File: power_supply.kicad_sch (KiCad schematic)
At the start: 16 parts, among them SW1 SW_DIP_x01, T1 1x230V 2x30V 300VA

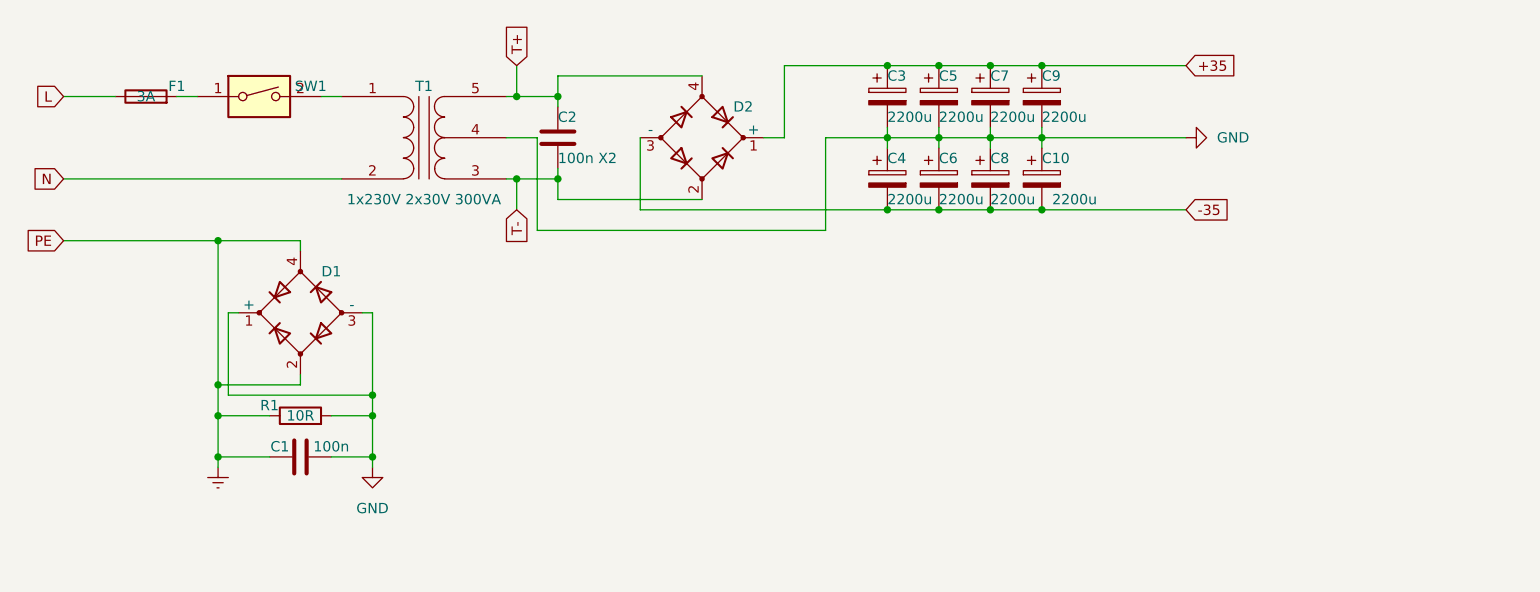
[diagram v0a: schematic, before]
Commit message: cosmetics
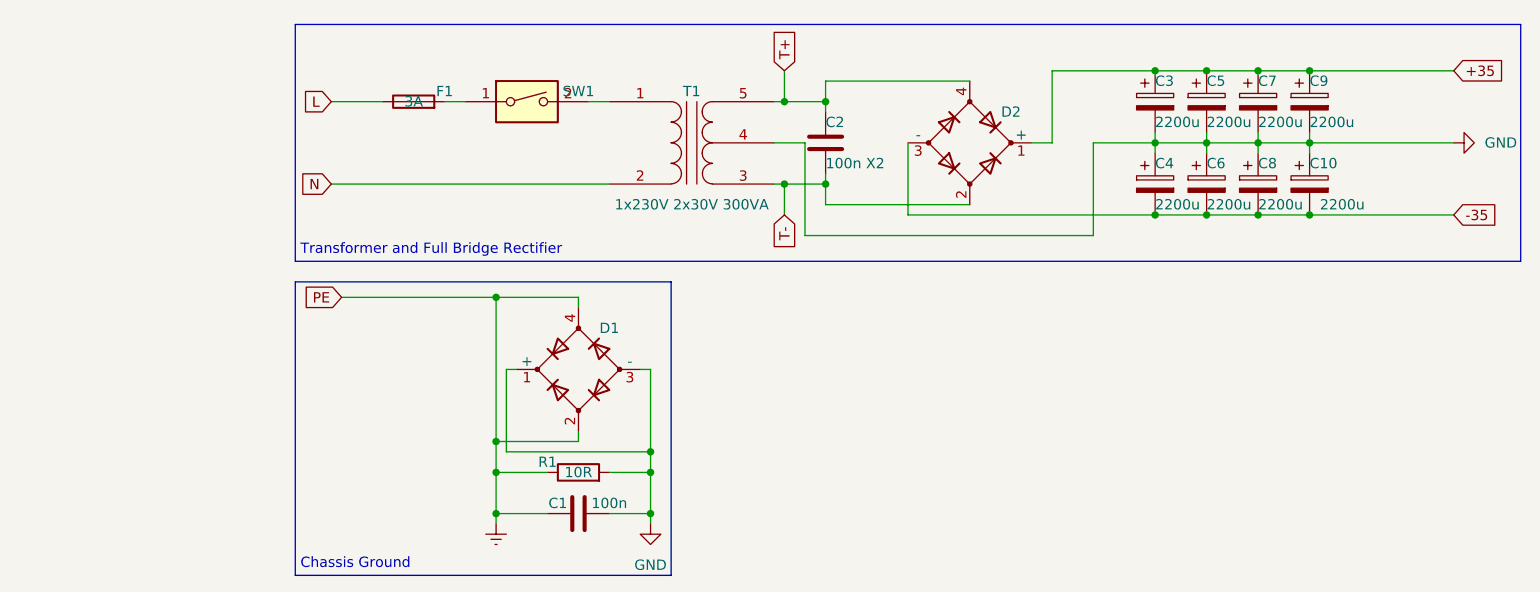
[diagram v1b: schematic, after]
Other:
- note added: "Chassis Ground"
- note added: "Transformer and Full Bridge Rectifier"
- moved on the sheet: C1, C10, C2, C3, C4, C5, C6, C7, C8, C9, D1, D2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
